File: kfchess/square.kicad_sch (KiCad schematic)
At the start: 14 parts, among them Q2 AO3400A

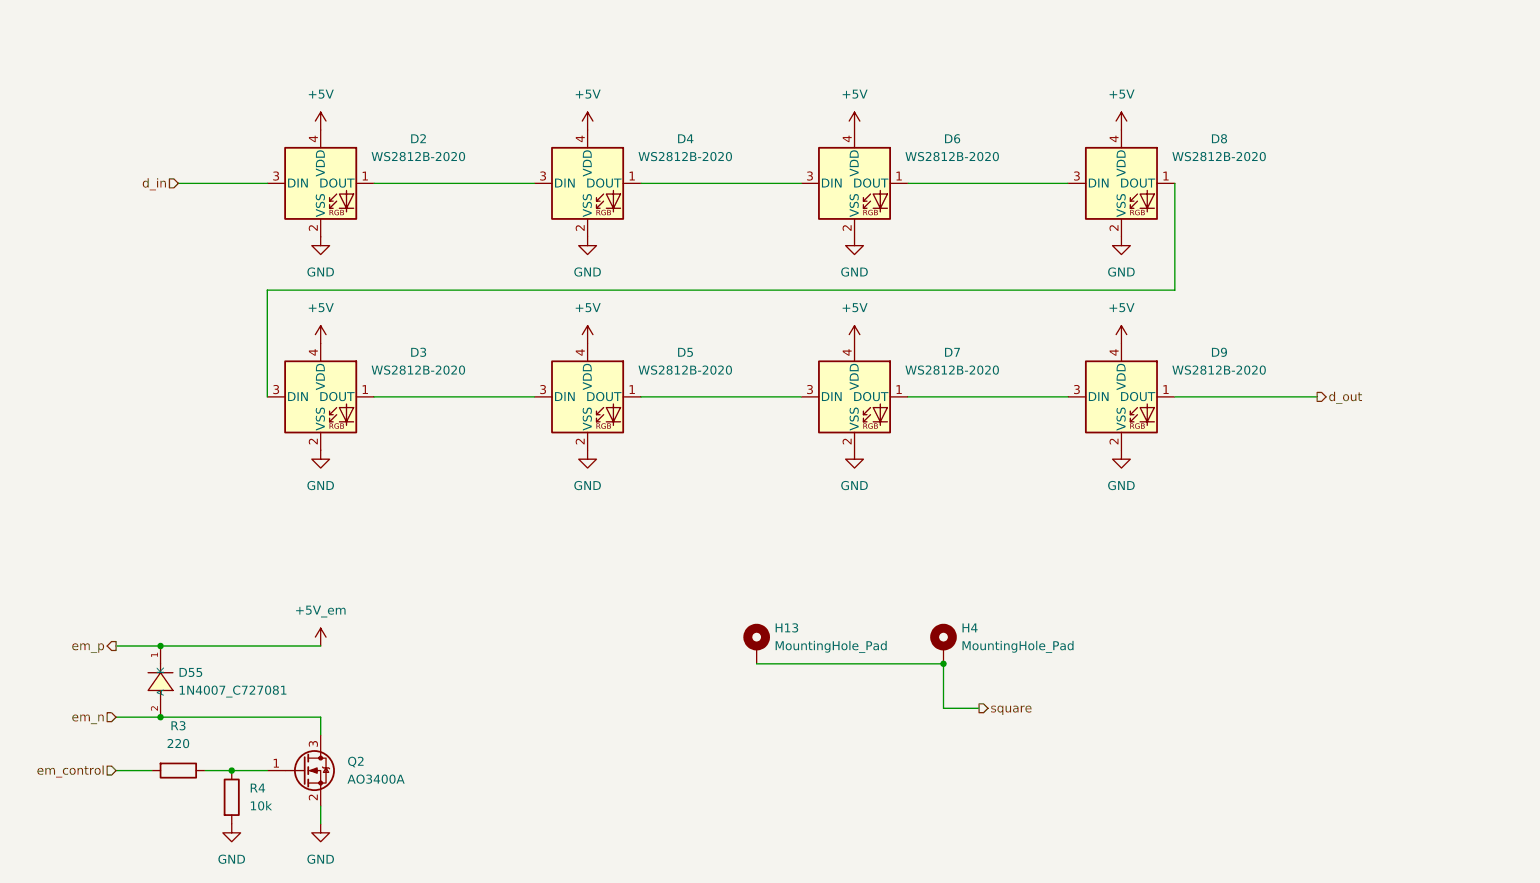
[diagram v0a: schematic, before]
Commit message: Started routing
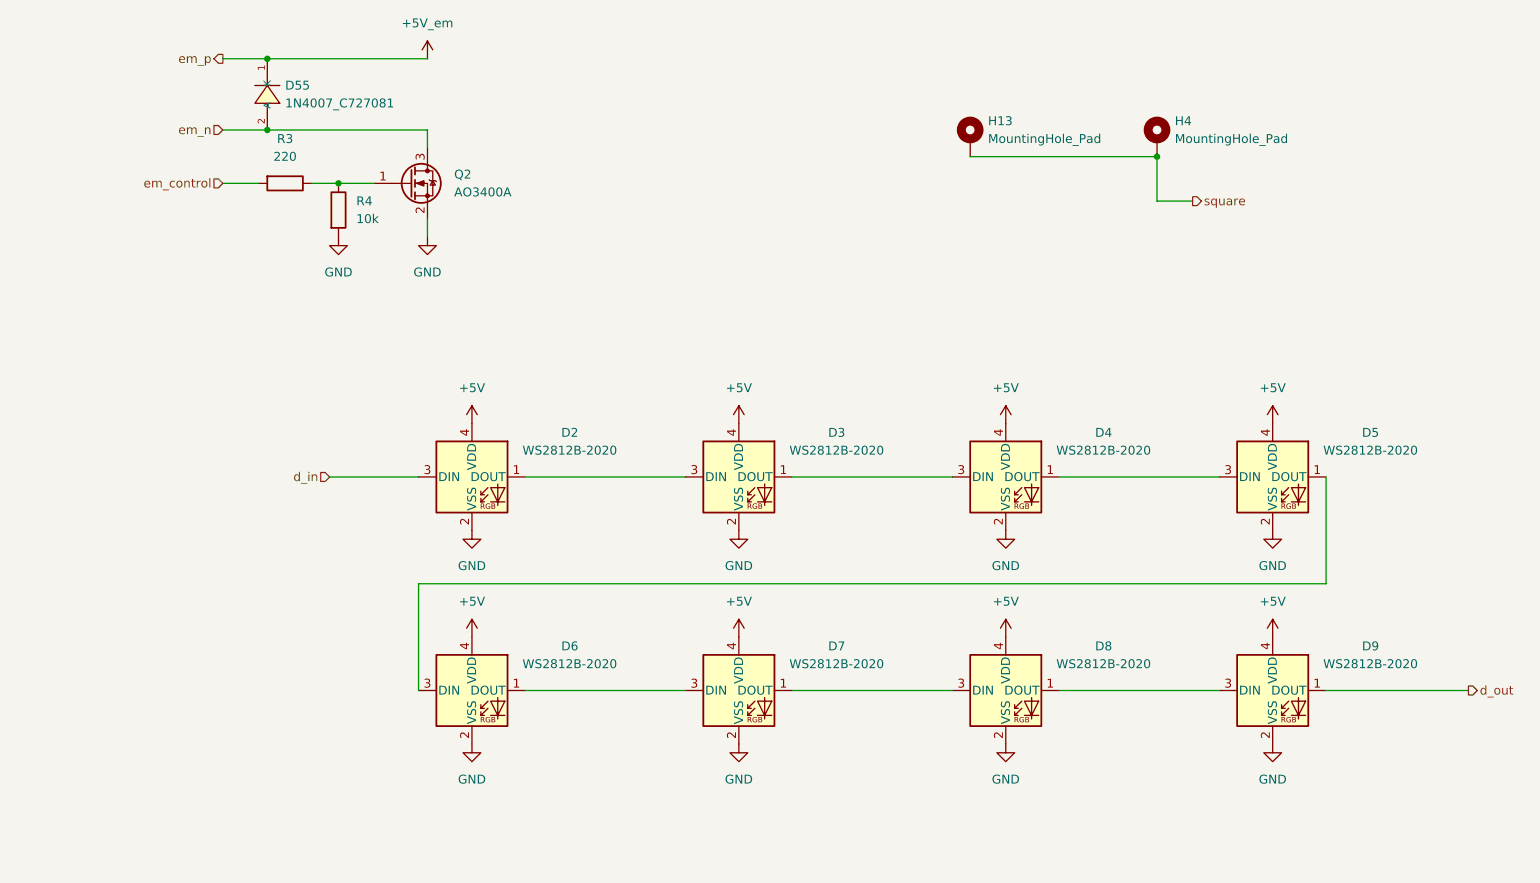
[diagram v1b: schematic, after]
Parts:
- renumbered D4 to D3, D6 to D4, D8 to D5, D3 to D6, D5 to D7, D7 to D8
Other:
- moved on the sheet: D2, D3, D4, D5, D55, D6, D7, D8, D9, H13, H4, Q2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
